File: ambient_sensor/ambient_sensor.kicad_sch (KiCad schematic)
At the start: 13 parts, among them J1 Conn_01x02_Pin, U4 ATmega328-P, U6 LD1117S33TR_SOT223, Y1 Crystal

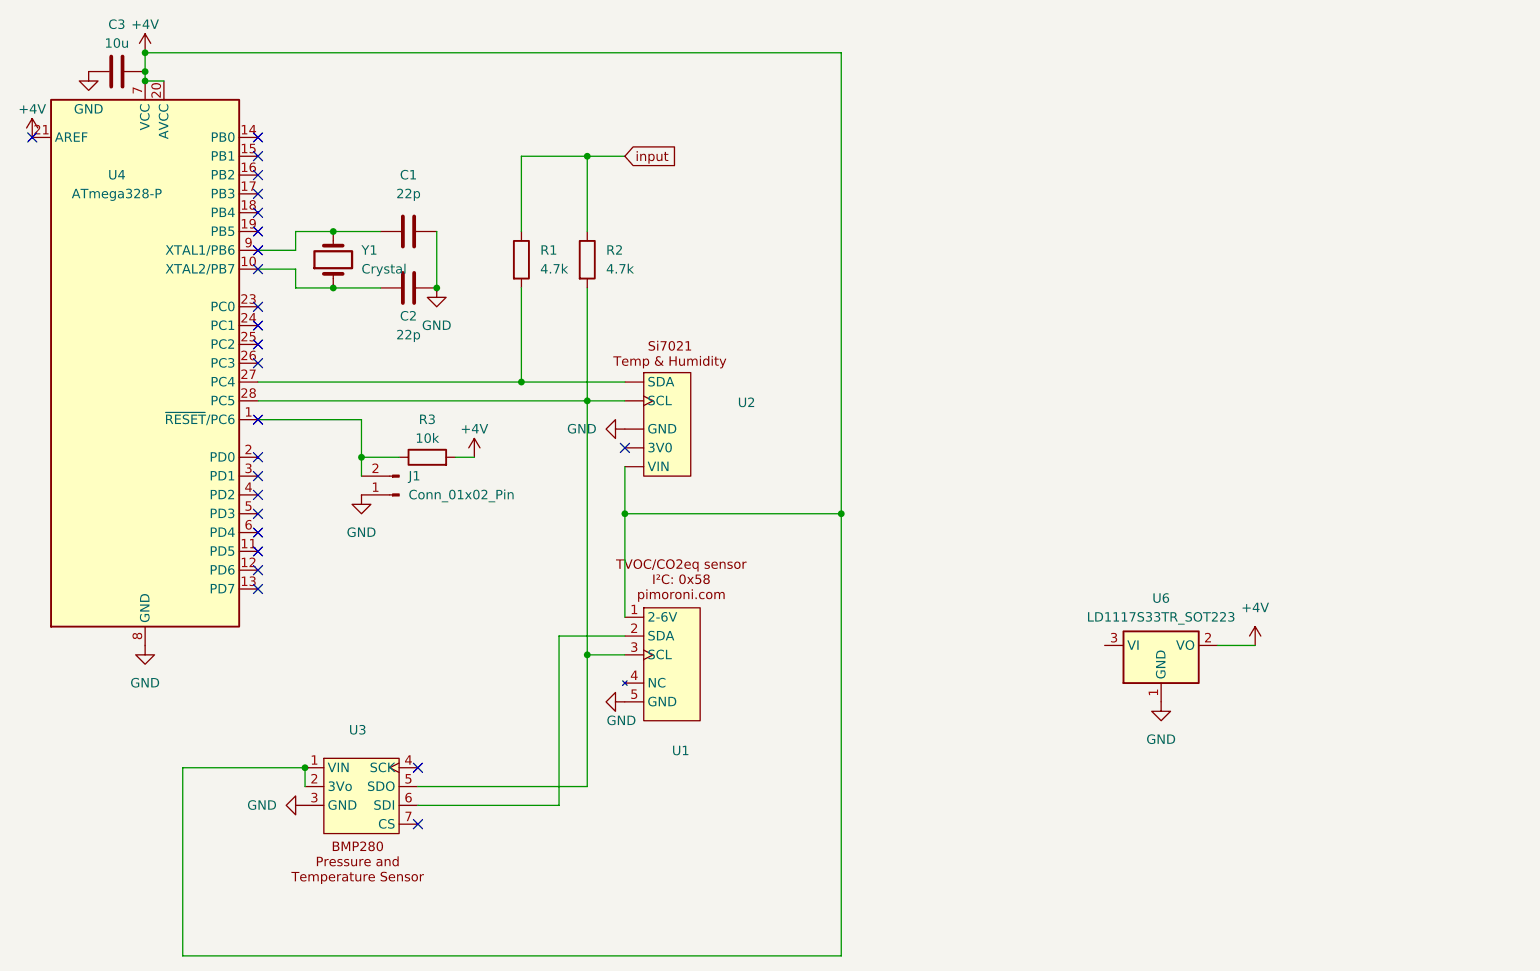
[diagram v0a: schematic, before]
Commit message: sensors connected
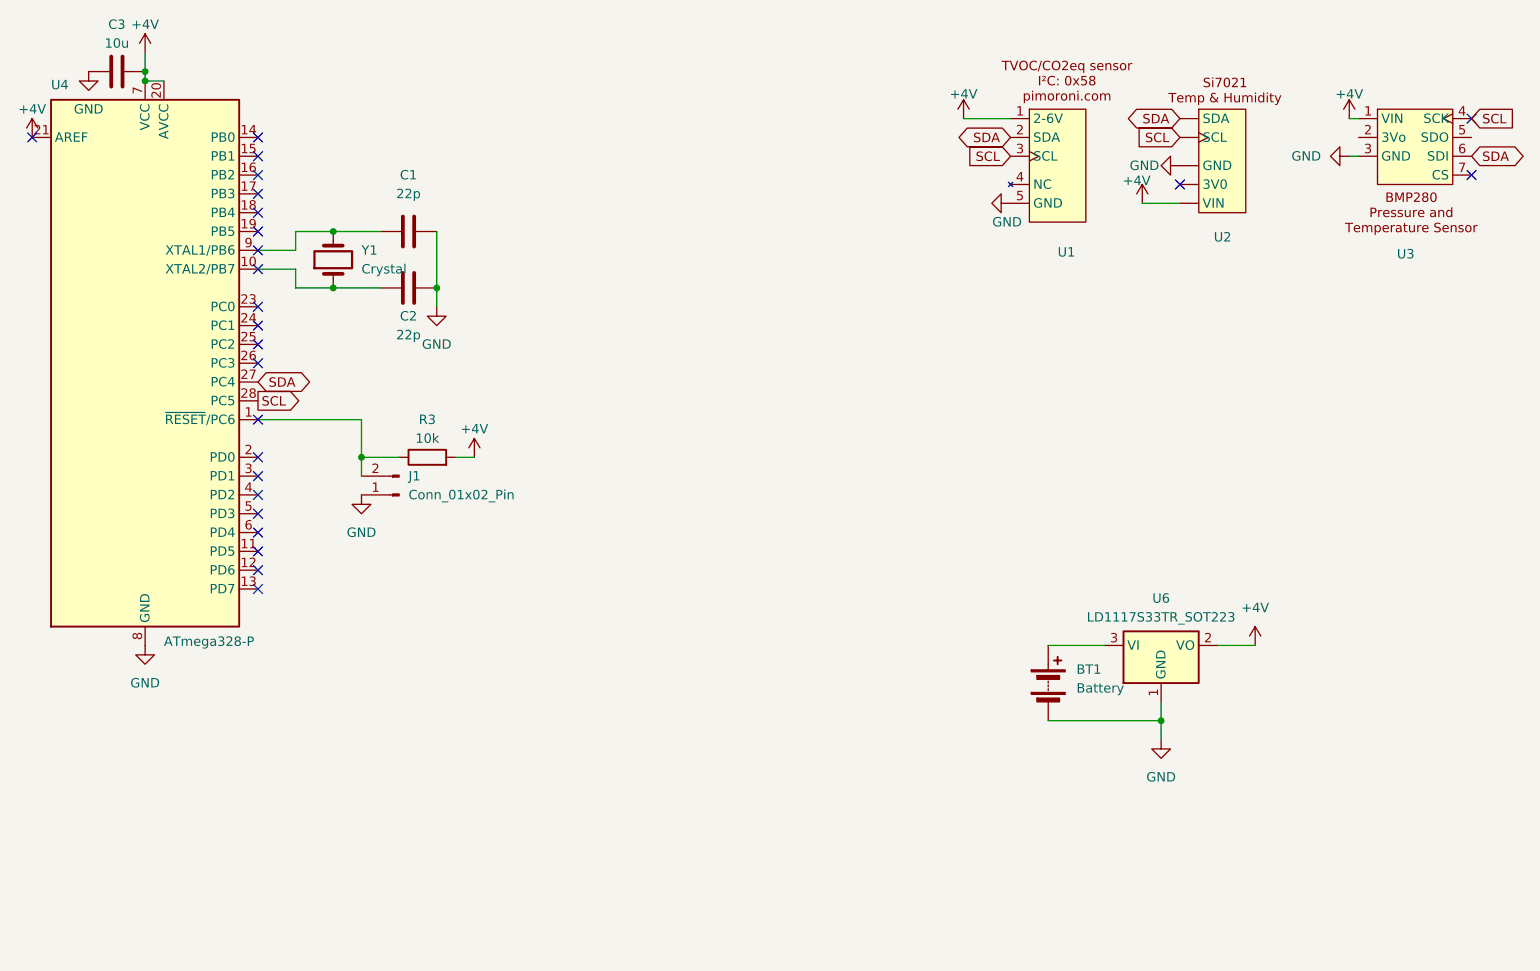
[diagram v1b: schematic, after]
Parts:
- removed R1: 4.7k, symbol Device:R
- removed R2: 4.7k, Resistor_SMD:R_1206_3216Metric, symbol Device:R
- added BT1: Battery, Battery:BatteryHolder_Keystone_2479_3xAAA, symbol Device:Battery
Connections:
- net +4V: no longer U3.2 (3Vo)
- net GND: now also BT1.2 (-)
- net SDA: now reaches U2. (VIN), U4.27 (PC4)
- net SDA: now also U1.2 (SDA), U3.6 (SDI)
- net SCL: now reaches U1.3 (SCL), U2. (VIN), U4.28 (PC5)
- net SCL: now also U3.4 (SCK); no longer U3.5 (SDO)
- net at U6.3 (VI): now also BT1.1 (+)
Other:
- moved on the sheet: U1, U2, U3
